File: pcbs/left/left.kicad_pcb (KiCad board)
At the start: 2 copper layers, 111.6 x 82.4 mm, 53 parts, among them J1 Conn_01x12_Socket

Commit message: fix offset etc
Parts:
- moved D1 200.0 mm to (96.5, 126.2)
- moved D10 200.0 mm to (127.0, 98.6)
- moved D11 200.0 mm to (127.0, 81.6)
- moved D12 200.0 mm to (145.0, 130.5)
- moved D13 200.0 mm to (145.0, 113.5)
- moved D14 200.0 mm to (145.0, 96.5)
- moved D15 200.0 mm to (145.0, 79.5)
- moved D16 200.0 mm to (163.0, 134.8)
- moved D17 200.0 mm to (163.0, 117.8)
- moved D18 200.0 mm to (163.0, 100.8)
- moved D19 200.0 mm to (163.0, 83.8)
- moved D2 200.0 mm to (91.0, 109.2)
- moved D20 200.0 mm to (180.2, 141.9)
- moved D21 200.0 mm to (181.0, 122.0)
- moved D22 200.0 mm to (181.0, 105.0)
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
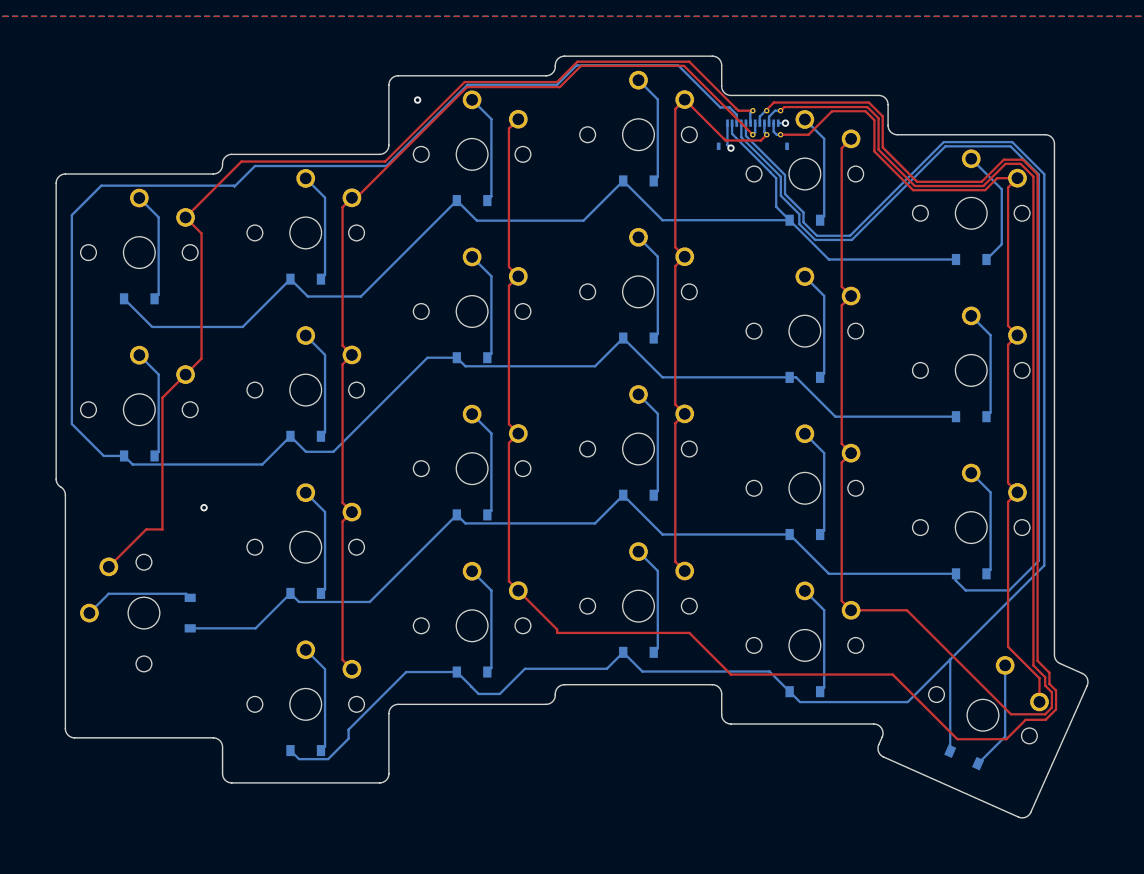
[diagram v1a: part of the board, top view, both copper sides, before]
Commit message: old changes
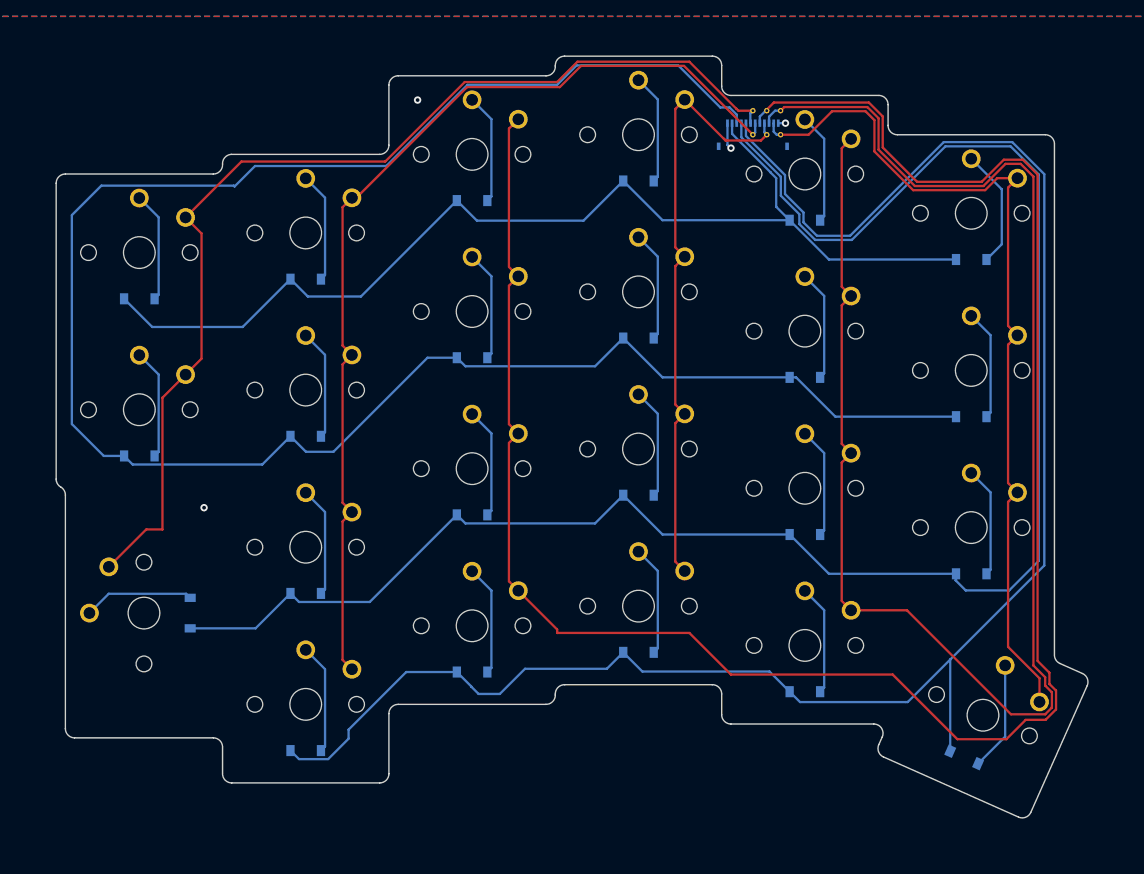
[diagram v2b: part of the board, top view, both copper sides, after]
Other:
- net class Default added: clearance 0.2, trace_width 0.25, via_dia 0.8, via_drill 0.4

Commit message: committing old changes
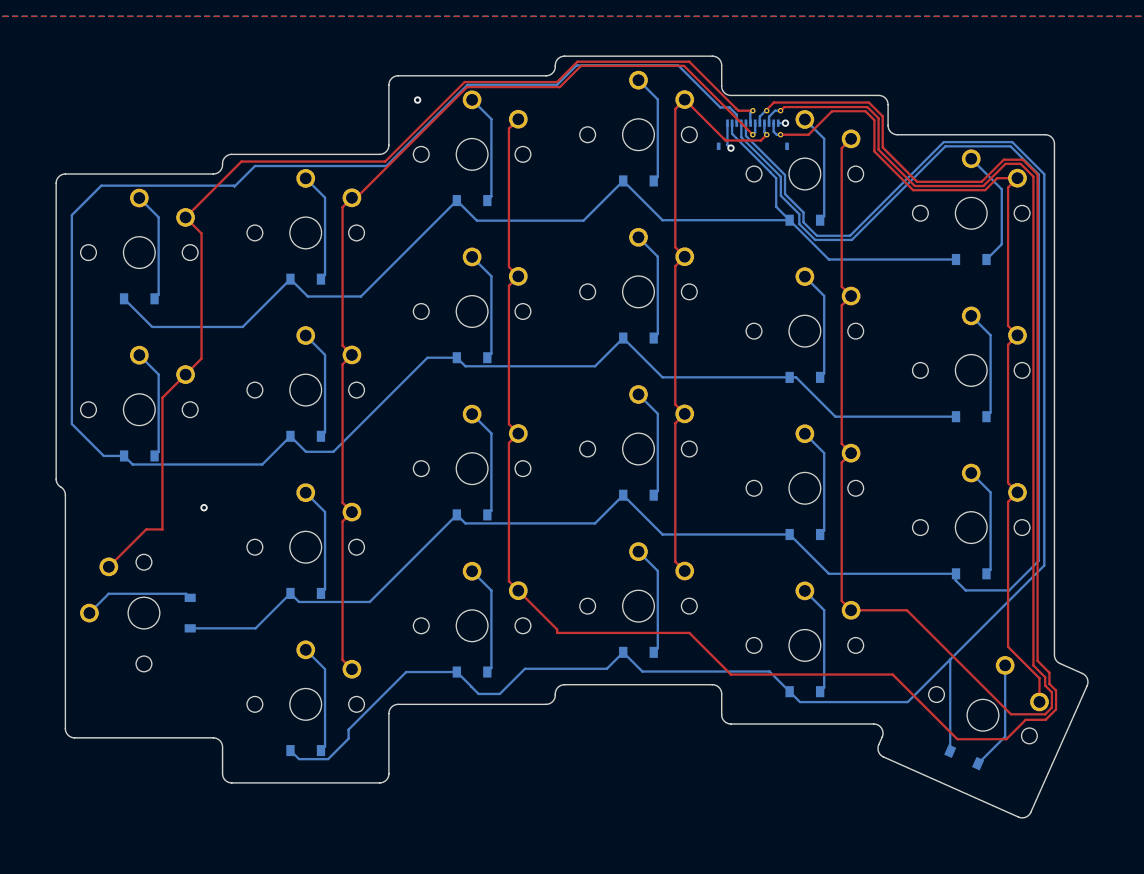
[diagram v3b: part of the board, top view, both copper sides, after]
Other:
- net class Default removed

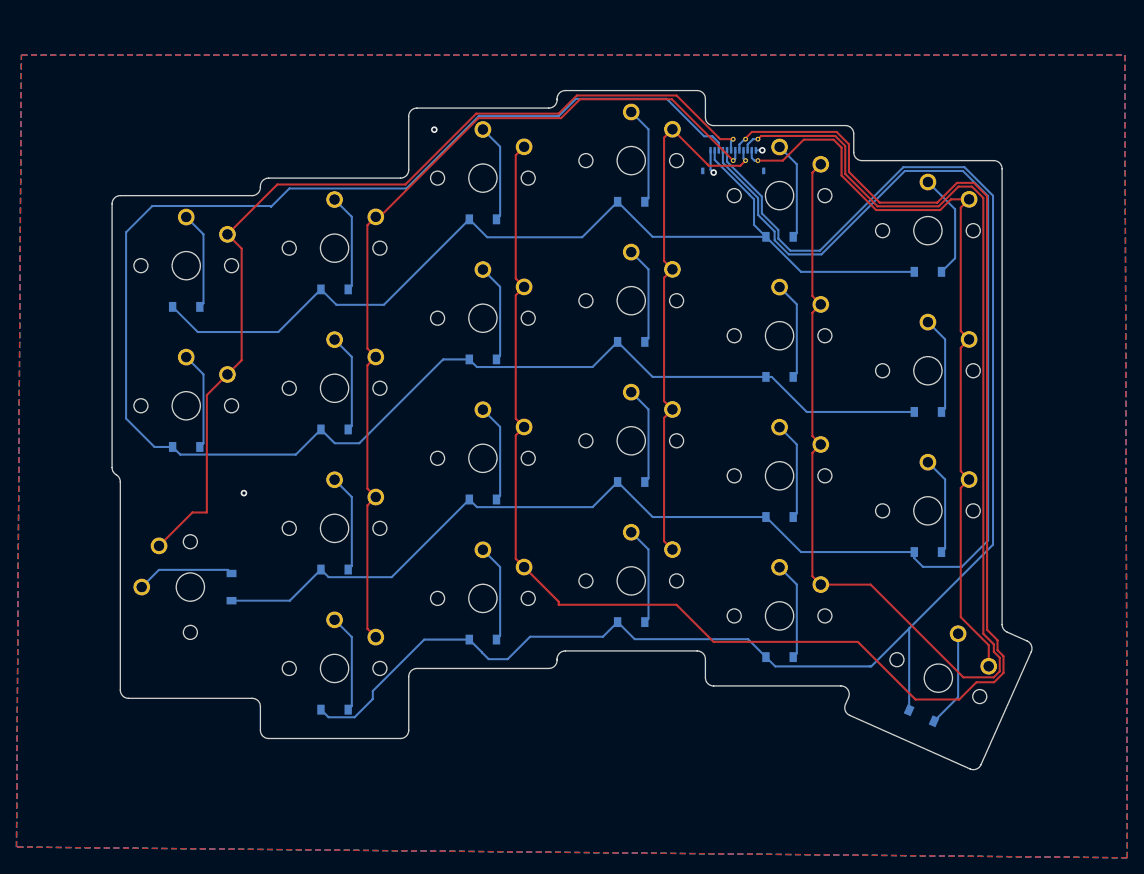
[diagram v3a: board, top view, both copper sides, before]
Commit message: lots of changes
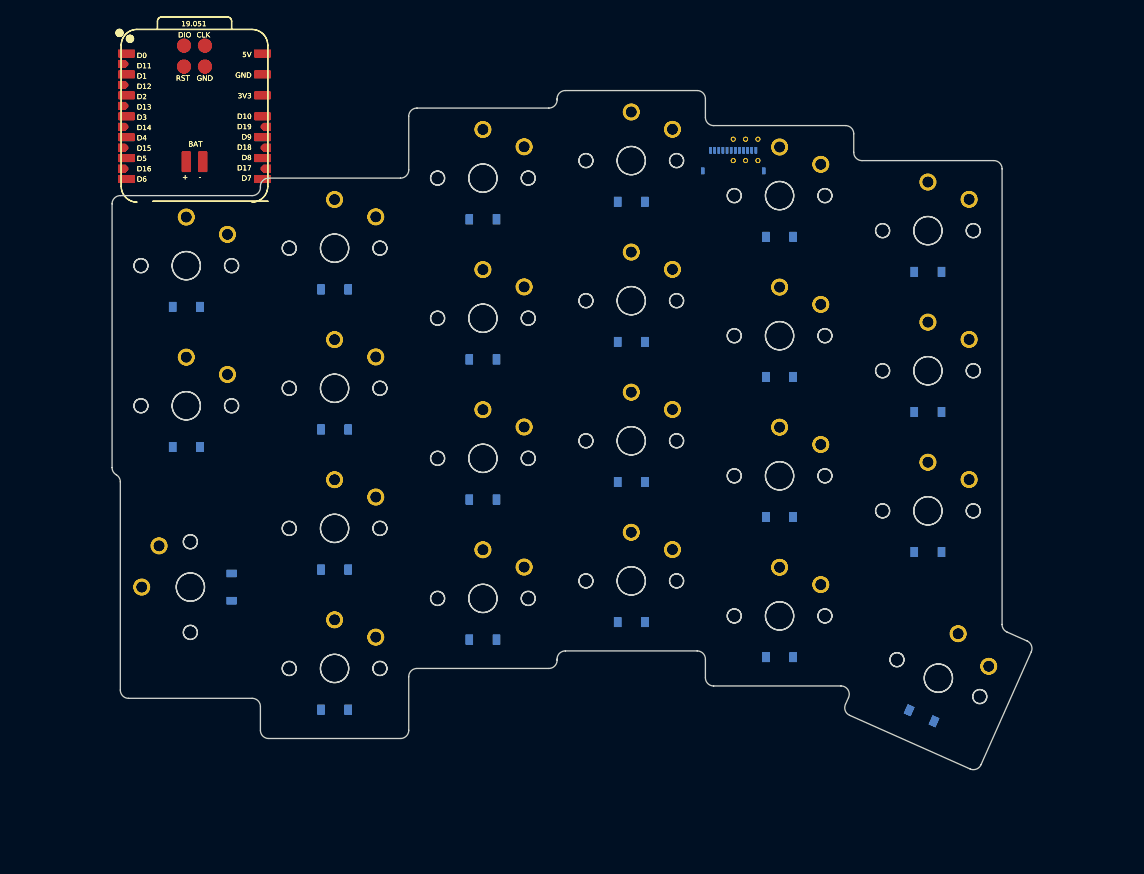
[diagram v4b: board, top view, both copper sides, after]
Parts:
- removed the D1 at (96.5, 126.2)
- removed the D10 at (127.0, 98.6)
- removed the D11 at (127.0, 81.6)
- removed the D12 at (145.0, 130.5)
- removed the D13 at (145.0, 113.5)
- removed the D14 at (145.0, 96.5)
- removed the D15 at (145.0, 79.5)
- removed the D16 at (163.0, 134.8)
- removed the D17 at (163.0, 117.8)
- removed the D18 at (163.0, 100.8)
- removed the D19 at (163.0, 83.8)
- removed the D2 at (91.0, 109.2)
- removed the D20 at (180.2, 141.9)
- removed the D21 at (181.0, 122.0)
- removed the D22 at (181.0, 105.0)
- removed the D23 at (181.0, 88.0)
- removed the D3 at (91.0, 92.2)
- removed the D4 at (109.0, 141.1)
- removed the D5 at (109.0, 124.1)
- removed the D6 at (109.0, 107.1)
- removed the D7 at (109.0, 90.1)
- removed the D8 at (127.0, 132.6)
- removed the D9 at (127.0, 115.6)
- removed the J1 at (157.4, 74.5)
- removed the S1 at (91.5, 126.2)
- removed the S10 at (127.0, 93.6)
- removed the S11 at (127.0, 76.6)
- removed the S12 at (145.0, 125.5)
- removed the S13 at (145.0, 108.5)
- removed the S14 at (145.0, 91.5)
- removed the S15 at (145.0, 74.5)
- removed the S16 at (163.0, 129.8)
- removed the S17 at (163.0, 112.8)
- removed the S18 at (163.0, 95.8)
- removed the S19 at (163.0, 78.8)
- removed the S2 at (91.0, 104.2)
- removed the S20 at (182.3, 137.3)
- removed the S21 at (181.0, 117.0)
- removed the S22 at (181.0, 100.0)
- removed the S23 at (181.0, 83.0)
- removed the S3 at (91.0, 87.2)
- removed the S4 at (109.0, 136.1)
- removed the S5 at (109.0, 119.1)
- removed the S6 at (109.0, 102.1)
- removed the S7 at (109.0, 85.1)
- removed the S8 at (127.0, 127.6)
- removed the S9 at (127.0, 110.6)
- removed the _1 at (157.4, 71.9)
- removed the _2 at (157.4, 74.5)
- removed the _3 at (158.9, 71.9)
- removed the _4 at (158.9, 74.5)
- removed the _5 at (160.4, 71.9)
- removed the _6 at (160.4, 74.5)
- added 19.051 (x2): , XIAO-nRF52840-Plus-SMD-updated, F.Cu at (91.0, 68.1)
- added D1 (x2): , ComboDiode, B.Cu at (96.5, 126.2)
- added D10 (x2): , ComboDiode, B.Cu at (127.0, 98.6)
- added D11 (x2): , ComboDiode, B.Cu at (127.0, 81.6)
- added D12 (x2): , ComboDiode, B.Cu at (145.0, 130.5)
- added D13 (x2): , ComboDiode, B.Cu at (145.0, 113.5)
- added D14 (x2): , ComboDiode, B.Cu at (145.0, 96.5)
- added D15 (x2): , ComboDiode, B.Cu at (145.0, 79.5)
- added D16 (x2): , ComboDiode, B.Cu at (163.0, 134.8)
- added D17 (x2): , ComboDiode, B.Cu at (163.0, 117.8)
- added D18 (x2): , ComboDiode, B.Cu at (163.0, 100.8)
- added D19 (x2): , ComboDiode, B.Cu at (163.0, 83.8)
- added D2 (x2): , ComboDiode, B.Cu at (91.0, 109.2)
- added D20 (x2): , ComboDiode, B.Cu at (180.2, 141.9)
- added D21 (x2): , ComboDiode, B.Cu at (181.0, 122.0)
- added D22 (x2): , ComboDiode, B.Cu at (181.0, 105.0)
- added D23 (x2): , ComboDiode, B.Cu at (181.0, 88.0)
- added D3 (x2): , ComboDiode, B.Cu at (91.0, 92.2)
- added D4 (x2): , ComboDiode, B.Cu at (109.0, 141.1)
- added D5 (x2): , ComboDiode, B.Cu at (109.0, 124.1)
- added D6 (x2): , ComboDiode, B.Cu at (109.0, 107.1)
- added D7 (x2): , ComboDiode, B.Cu at (109.0, 90.1)
- added D8 (x2): , ComboDiode, B.Cu at (127.0, 132.6)
- added D9 (x2): , ComboDiode, B.Cu at (127.0, 115.6)
- added J1 (x2): Conn_01x12_Socket, GCT_FFC2B28-12-G, B.Cu at (157.4, 74.5)
- added S1 (x2): , PG1350, F.Cu at (91.5, 126.2)
- added S10 (x2): , PG1350, F.Cu at (127.0, 93.6)
- added S11 (x2): , PG1350, F.Cu at (127.0, 76.6)
- added S12 (x2): , PG1350, F.Cu at (145.0, 125.5)
- added S13 (x2): , PG1350, F.Cu at (145.0, 108.5)
- added S14 (x2): , PG1350, F.Cu at (145.0, 91.5)
- added S15 (x2): , PG1350, F.Cu at (145.0, 74.5)
- added S16 (x2): , PG1350, F.Cu at (163.0, 129.8)
- added S17 (x2): , PG1350, F.Cu at (163.0, 112.8)
- added S18 (x2): , PG1350, F.Cu at (163.0, 95.8)
- added S19 (x2): , PG1350, F.Cu at (163.0, 78.8)
- added S2 (x2): , PG1350, F.Cu at (91.0, 104.2)
- added S20 (x2): , PG1350, F.Cu at (182.3, 137.3)
- added S21 (x2): , PG1350, F.Cu at (181.0, 117.0)
- added S22 (x2): , PG1350, F.Cu at (181.0, 100.0)
- added S23 (x2): , PG1350, F.Cu at (181.0, 83.0)
- added S3 (x2): , PG1350, F.Cu at (91.0, 87.2)
- added S4 (x2): , PG1350, F.Cu at (109.0, 136.1)
- added S5 (x2): , PG1350, F.Cu at (109.0, 119.1)
- added S6 (x2): , PG1350, F.Cu at (109.0, 102.1)
- added S7 (x2): , PG1350, F.Cu at (109.0, 85.1)
- added S8 (x2): , PG1350, F.Cu at (127.0, 127.6)
- added S9 (x2): , PG1350, F.Cu at (127.0, 110.6)
- added _1 (x2): VIA-0.6mm, VIA-0.6mm, F.Cu at (157.4, 71.9)
- added _2 (x2): VIA-0.6mm, VIA-0.6mm, F.Cu at (157.4, 74.5)
- added _3 (x2): VIA-0.6mm, VIA-0.6mm, F.Cu at (158.9, 71.9)
- added _4 (x2): VIA-0.6mm, VIA-0.6mm, F.Cu at (158.9, 74.5)
- added _5 (x2): VIA-0.6mm, VIA-0.6mm, F.Cu at (160.4, 71.9)
- added _6 (x2): VIA-0.6mm, VIA-0.6mm, F.Cu at (160.4, 74.5)
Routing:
- net C3: track 217.2 -> 0.00 mm
- net R3: track 213.2 -> 0.00 mm
- net R1: track 195.5 -> 0.00 mm
- net R2: track 192.7 -> 0.00 mm
- net C5: track 175.3 -> 0.00 mm
- net R4: track 117.8 -> 0.00 mm
- net C1: track 115.7 -> 0.00 mm
- net C2: track 107.2 -> 0.00 mm
- net C6: track 94.8 -> 0.00 mm
- net C4: track 66.1 -> 0.00 mm
- net inner_top: track 13.0 -> 0.00 mm
- net pinky_top: track 11.9 -> 0.00 mm
- net pinky_middle: track 11.9 -> 0.00 mm
- net pinky_bottom: track 11.9 -> 0.00 mm
- net outerleft_top: track 11.9 -> 0.00 mm
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- removed copper zone on B.Cu, net GND
- removed copper zone on F.Cu, net GND
